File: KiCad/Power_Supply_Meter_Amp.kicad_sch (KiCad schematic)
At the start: 637 parts, among them J1 R_Phono_In, J10 VCC_IN, J11 VCC_OUT, J12 EMK_In, J15 Mic_Effekt_Out, J16 Mic_Effekt_Out, J17 Mic_Effekt_Out, J18 Mic_Effekt_Out, J19 Phono/Line_Out, J2 L_Phono_In, J20 Mic_Effekt_Out, J21 Conn_01x05_bridged, J22 EMK_In, J24 Mic_Effekt_In, J25 Mic_Effekt_In, J26 Phono/Line_In, J27 Mic_Effekt_In, J28 Pegel_Out, J29 Pegel_Out, J3 R_Line_In, J30 Pegel_In, J31 Pegel_In, J32 Pegel_In, J33 Pegel_In, J34 LED_Out, J35 LED_In, J36 VU_Meter_Out, J37 AUX_Send_3, J38 AUX_Send_1, J39 AUX_Send_2, J4 L_Line_In, J40 Bass_Out, J41 Kick_Out, J42 Mid_Out, J43 High_Out, J44 Line_Out_L, J45 Line_Out_R, J5 Mic_In, J6 Effekt_In, J7 AUX_RET_1, J8 AUX_RET_2, J9 AUX_RET_3, SW1 SW_DPST, SW10 SW_SPDT, SW11 SW_SPDT, SW12 SW_SPDT, SW2 SW_SPDT, SW3 SW_SPDT, SW4 SW_SPDT, SW5 SW_SPDT, SW6 SW_SPDT, SW7 SW_SPDT, SW8 SW_SPDT, SW9 SW_Rotary_1x4, U1 TL074, U10 TL074, U11 TL074, U12 TL074, U13 TL074, U14 TL074, U15 TL074, U16 TL074, U17 TL074, U18 TL074, U19 TL074, U2 TL074, U20 TL074, U21 TL074, U22 TL074, U23 TL074, U24 TL074, U25 INA128U, U3 TL074, U4 TL074, U5 TL074, U6 REC10K-2409, U7 REC10K-2415, U8 TL074, U9 TL074

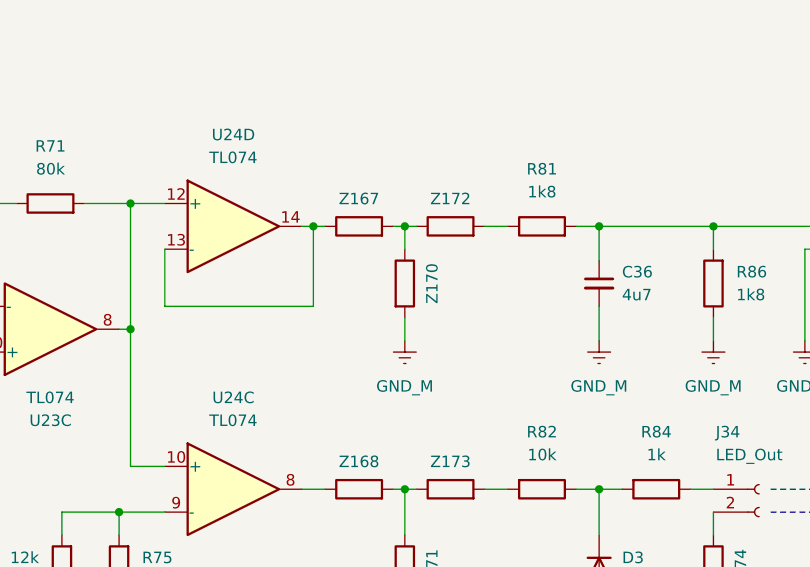
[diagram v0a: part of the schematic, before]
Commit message: PCB Update
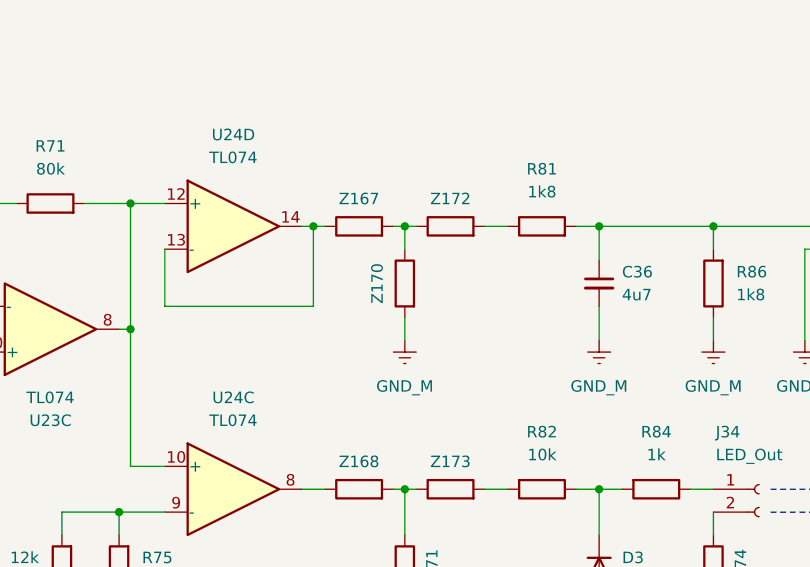
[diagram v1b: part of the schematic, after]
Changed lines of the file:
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@@
 	(wire
 		(pts
+			(xy 637.54 518.16) (xy 650.24 518.16)
+		)
+		(stroke
+			(width 0)
+			(type default)
+		)
+	)
+	(wire
+		(pts
 			(xy 781.05 105.41) (xy 781.05 104.14)
 		)
@@
 	(wire
 		(pts
-			(xy 637.54 518.16) (xy 650.24 518.16)
-		)
-		(stroke
-			(width 0)
-			(type default)
-		)
-	)
-	(wire
-		(pts
 			(xy 487.68 283.21) (xy 490.22 283.21)
 		)
@@
 		(lib_id "Device:R")
 		(at 584.2 519.43 0)
+		(mirror y)
 		(unit 1)
 		(exclude_from_sim no)
@@
 		(dnp no)
 		(property "Reference" "Z170"
-			(at 587.248 519.43 90)
+			(at 581.152 519.43 90)
 			(effects
 				(font
@@
 		)
 		(property "Value" "~"
-			(at 588.01 519.43 90)
+			(at 580.39 519.43 90)
 			(effects
 				(font
@@
 		)
 		(property "Footprint" "Resistor_SMD:R_0805_2012Metric_Pad1.20x1.40mm_HandSolder"
-			(at 582.422 519.43 90)
+			(at 585.978 519.43 90)
 			(effects
 				(font
@@
 		(on_board yes)
 		(dnp no)
-		(fields_autoplaced yes)
 		(property "Reference" "R75"
 			(at 554.99 549.9099 0)
